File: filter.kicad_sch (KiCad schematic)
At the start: 93 parts, among them U1 ${SIM.PARAMS}

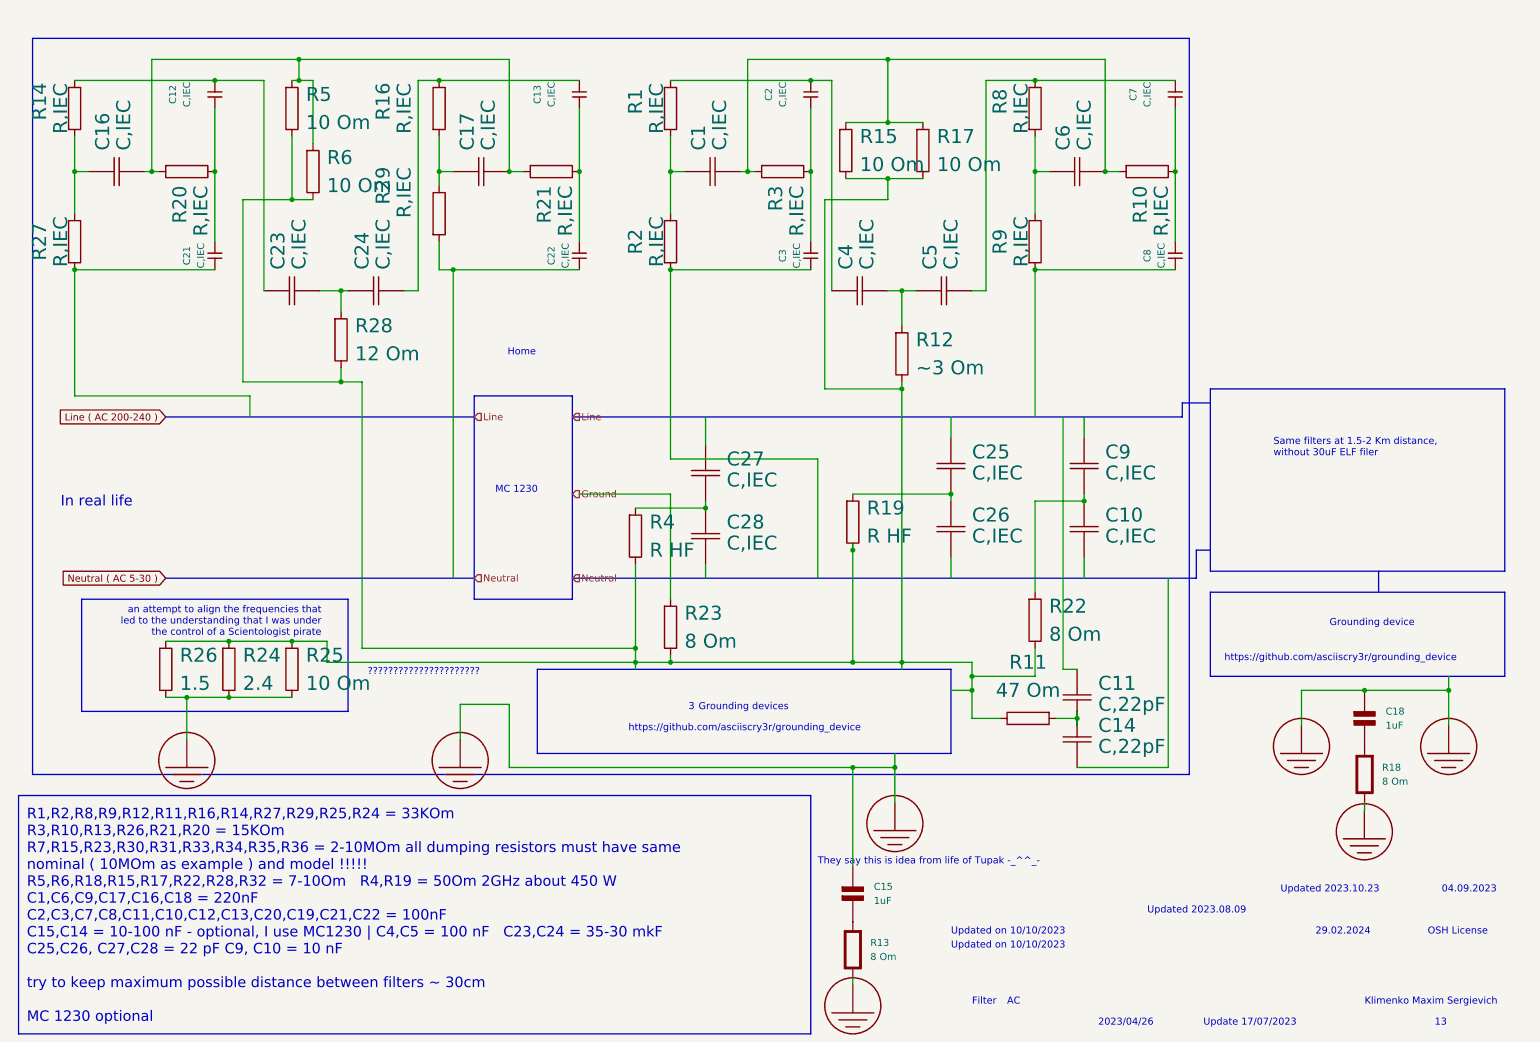
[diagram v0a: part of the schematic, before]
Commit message: Upgrade
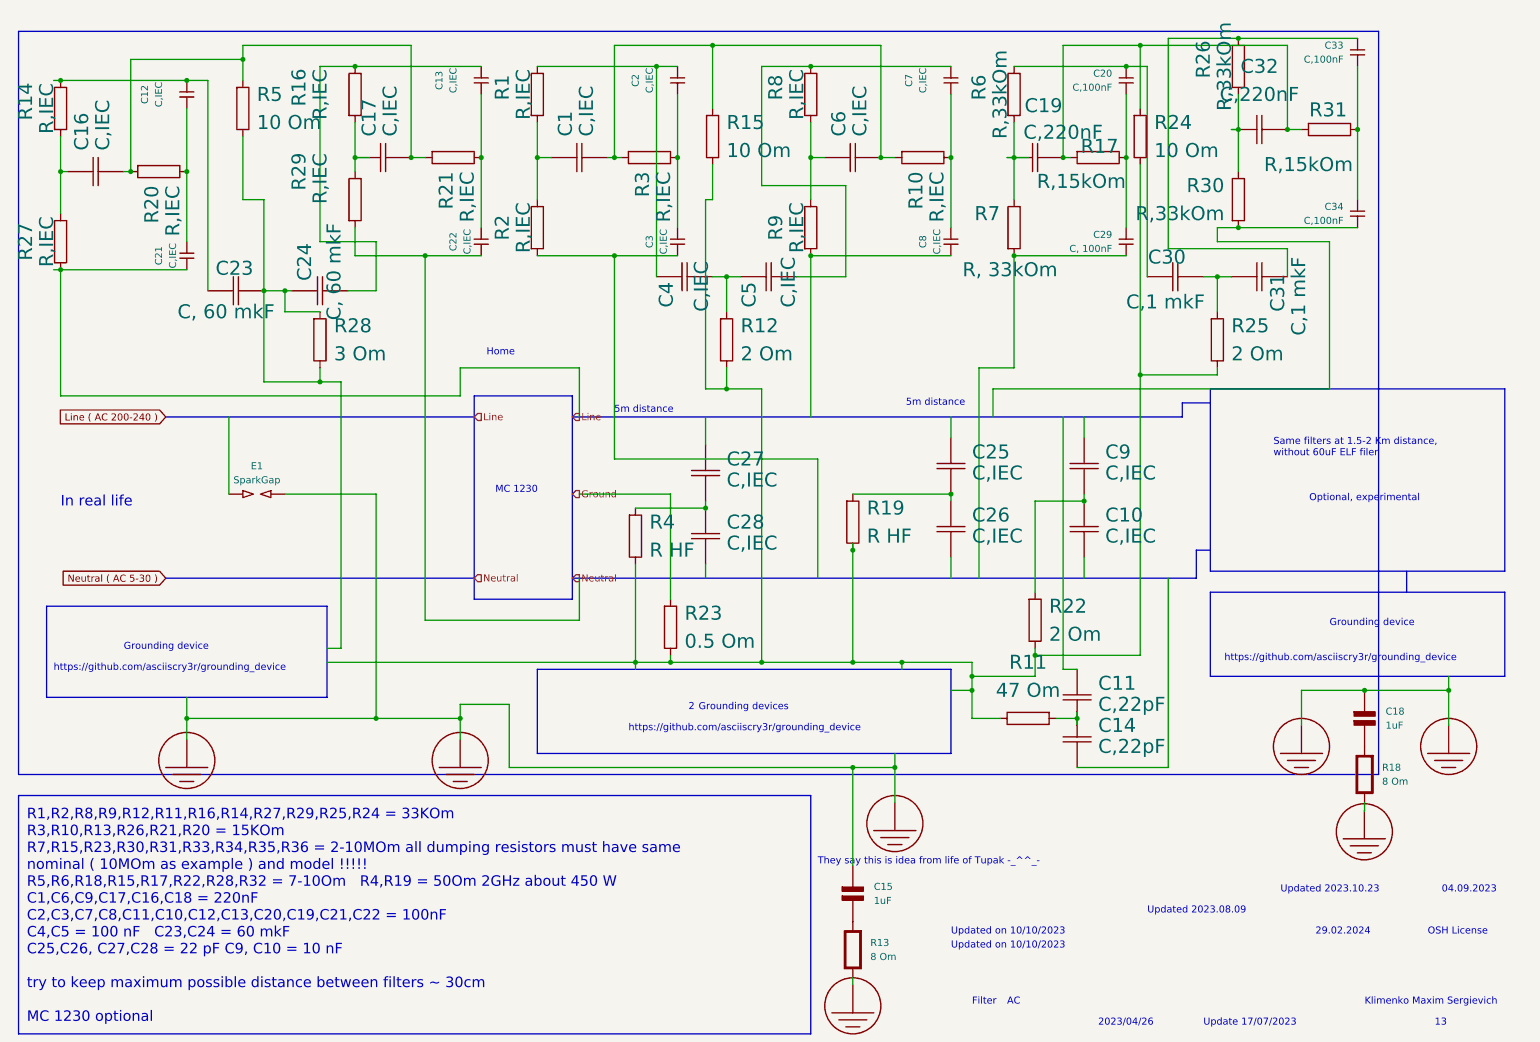
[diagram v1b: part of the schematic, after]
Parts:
- added C19, C32: C,220nF, symbol PCM_Generic:C,IEC
- added C20, C33, C34: C,100nF, symbol PCM_Generic-50:C,IEC
- added C29: C, 100nF, symbol PCM_Generic-50:C,IEC
- added C30, C31: C,1 mkF, symbol PCM_Generic:C,IEC
- added E1: SparkGap, symbol Device:SparkGap
- added R30: R,33kOm, symbol PCM_Generic:R,IEC
- added R31: R,15kOm, symbol PCM_Generic:R,IEC
- added R7: R, 33kOm, symbol PCM_Generic:R,IEC
- C23, C24: value C,IEC -> C, 60 mkF
- R12: value ~3 Om -> 2 Om
- R17: value 10 Om -> R,15kOm; Indicator (none) -> +
- R22: value 8 Om -> 2 Om
- R23: value 8 Om -> 0.5 Om
- R24: value 2.4 -> 10 Om
- R25: value 10 Om -> 2 Om
- R26: value 1.5 -> R,33kOm; Indicator (none) -> +
- R28: value 12 Om -> 3 Om
- R6: value 10 Om -> R,33kOm; Indicator (none) -> +
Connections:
- net PE: now also E1.2; no longer R24.2 (-), R25.2 (-), R26.2 (-)
- net at C23.2 (-), C24.1 (+), R28.1 (+): now also R28.2 (-), R5.2 (-)
- net at C16.2 (-), C17.2 (-), R20.1 (+)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: no longer R6.1 (+)
- net at C1.2 (-), C6.2 (-), R10.1 (+)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: no longer R17.1 (+)
- net at R11.2 (-), R12.2 (-), R15.2 (-)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: now also R24.2 (-), R25.2 (-); no longer R17.2 (-), R24.1 (+), R25.1 (+), R26.1 (+), R28.2 (-), R5.2 (-), R6.2 (-)
- new net: C19.2 (-), C32.2 (-), R17.1 (+), R24.1 (+), R31.1 (+)
- new net: C33.1 (+), C34.2 (-), R31.2 (-)
- new net: C20.2 (-), C30.1 (+), R6.2 (-)
- new net: C30.2 (-), C31.1 (+), R25.1 (+)
- new net: C31.2 (-), C33.2 (-), R26.2 (-)
- new net: C29.1 (+), R7.1 (+)
- new net: C20.1 (+), C29.2 (-), R17.2 (-)
- new net: C19.1 (+), R6.1 (+), R7.2 (-)
- new net: C34.1 (+), R30.1 (+)
- new net: C32.1 (+), R26.1 (+), R30.2 (-)
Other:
- note added: "2"
- note added: "5m distance"
- note added: "Optional, experimental"
- note added: "Same filters at 1.5-2 Km distance, without 60uF ELF filer"
- note removed: "3"
- note removed: "??????????????????????"
- note removed: "Same filters at 1.5-2 Km distance, without 30uF ELF filer"
- note removed: "an attempt to align the frequencies that led to the understanding that I was under the control of a Scientologist pirate"
- moved on the sheet: C1, C12, C13, C16, C17, C2, C21, C22, C23, C24, C3, C4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
